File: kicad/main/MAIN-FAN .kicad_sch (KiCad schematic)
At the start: 8 parts, among them Q1 2302V

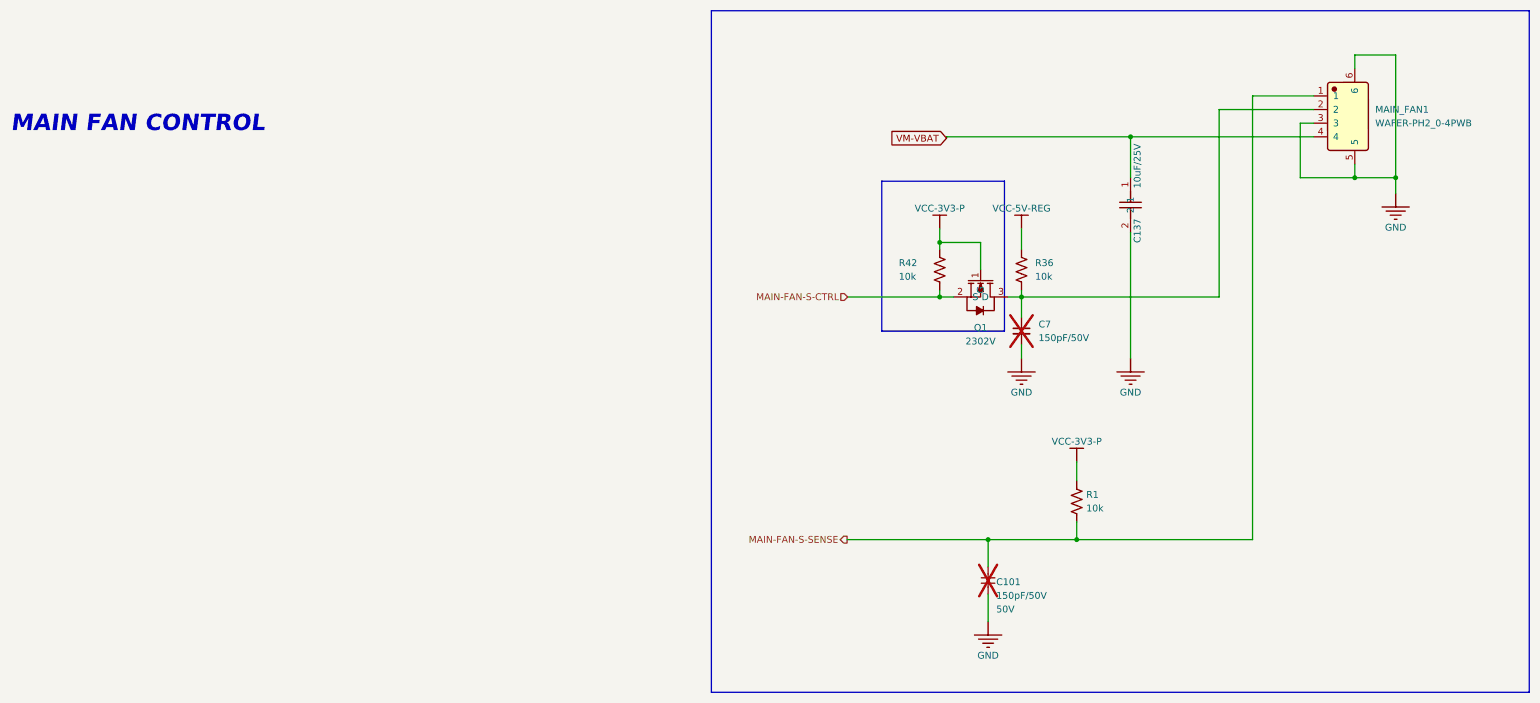
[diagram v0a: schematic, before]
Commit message: Second review round
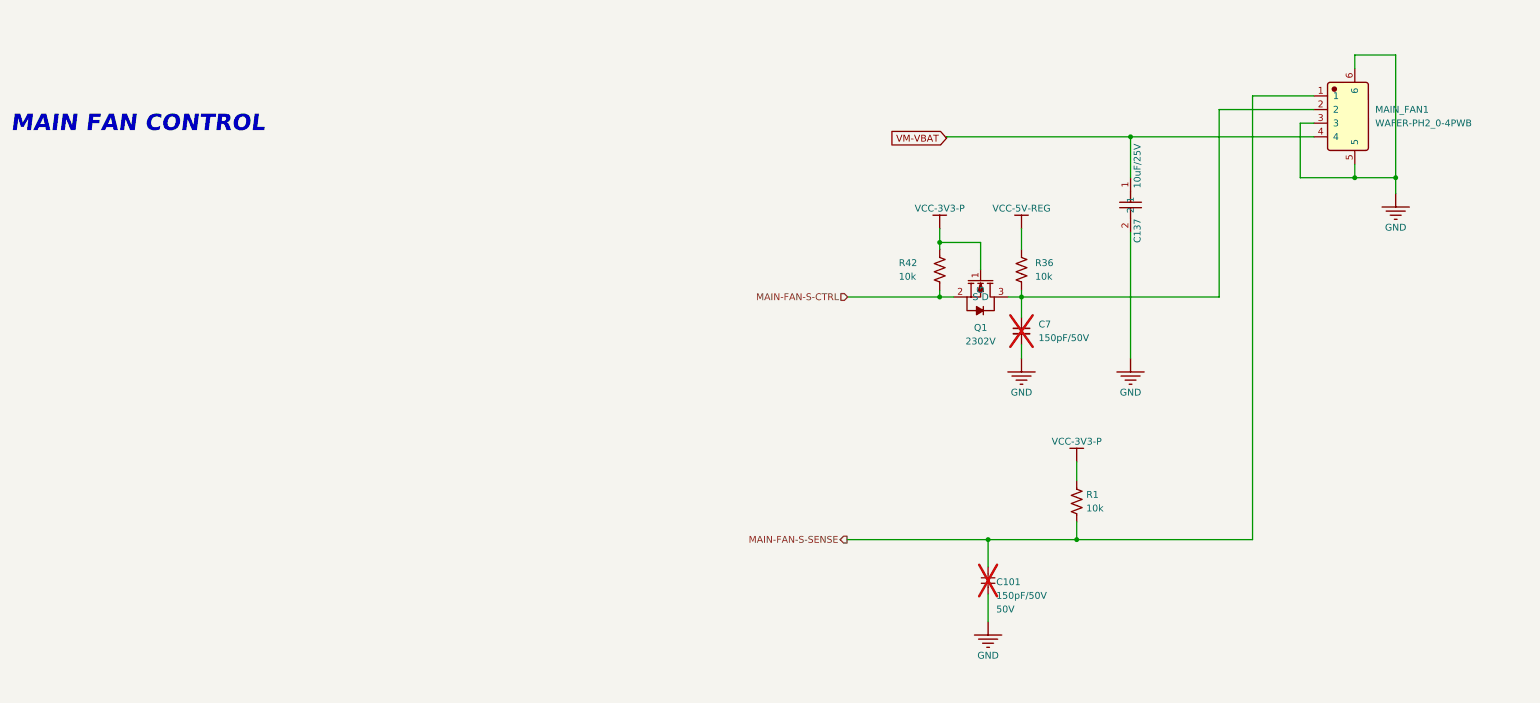
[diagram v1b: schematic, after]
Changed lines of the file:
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@@
 	(generator_version "10.0")
 	(paper "A2")
-	(rectangle
-		(start 308.61 106.68)
-		(end 461.01 233.68)
-		(stroke
-			(width 0)
-			(type solid)
-		)
-		(fill
-			(type color)
-			(color 0 72 0 1)
-		)
-	)
-	(rectangle
-		(start 340.36 138.43)
-		(end 363.22 166.37)
-		(stroke
-			(width 0)
-			(type solid)
-		)
-		(fill
-			(type color)
-			(color 132 0 0 1)
-		)
-	)
 	(text "MAIN FAN CONTROL"
 		(exclude_from_sim no)

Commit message: STM32 power rail switch
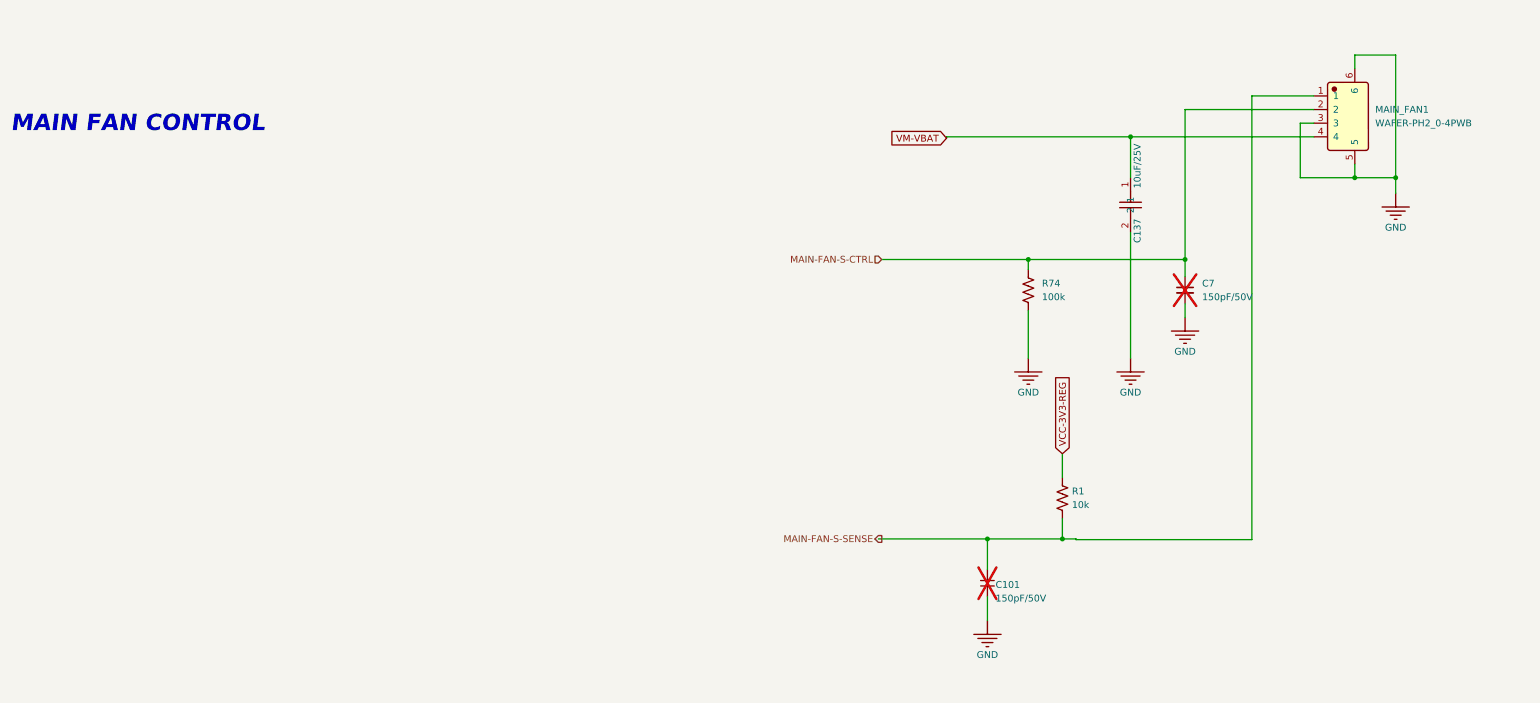
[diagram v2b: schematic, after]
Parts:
- removed Q1: 2302V, JLCImport:2302V, symbol JLCImport:2302V
- removed R36, R42: 10k, Resistor_SMD:R_0603_1608Metric, symbol Device:R_US
- added R74: 100k, Resistor_SMD:R_0603_1608Metric, symbol Device:R_US
- C101: LCSC (none) -> C107075; VOLTAGERATE 50V -> (none)
- C7: LCSC (none) -> C107075
- R1: LCSC (none) -> C98220
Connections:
- net GND: now also R74.2
- net MAIN-FAN-S-CTRL: now also C7.1, MAIN_FAN1.2, R74.1
- net VCC-3V3-P renamed VCC-3V3-REG
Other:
- moved on the sheet: C101, C7, R1
